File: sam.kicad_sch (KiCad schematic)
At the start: 59 parts, among them IC1 HYB4116, IC15 MC6883, IC16 74LS244N, IC2 HYB4116, IC3 HYB4116, IC31 74LS02N, IC33 74LS138N, IC4 HYB4116, IC5 HYB4116, IC6 HYB4116, IC7 HYB4116, IC8 HYB4116

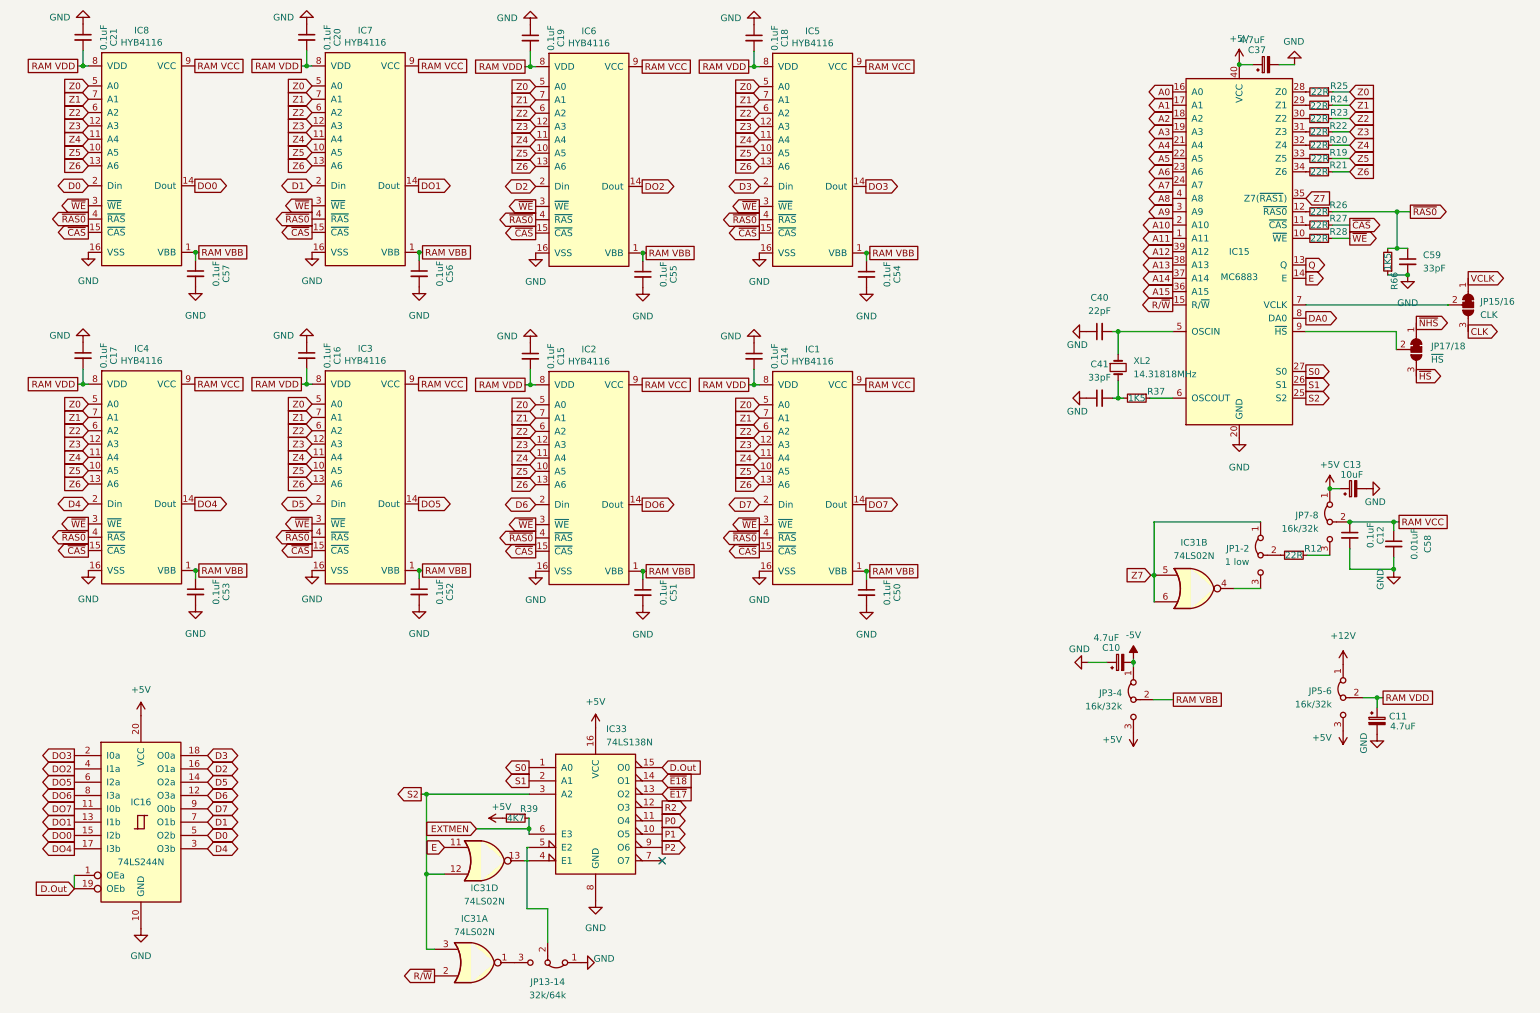
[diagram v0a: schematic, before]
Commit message: update board for revision 2.2
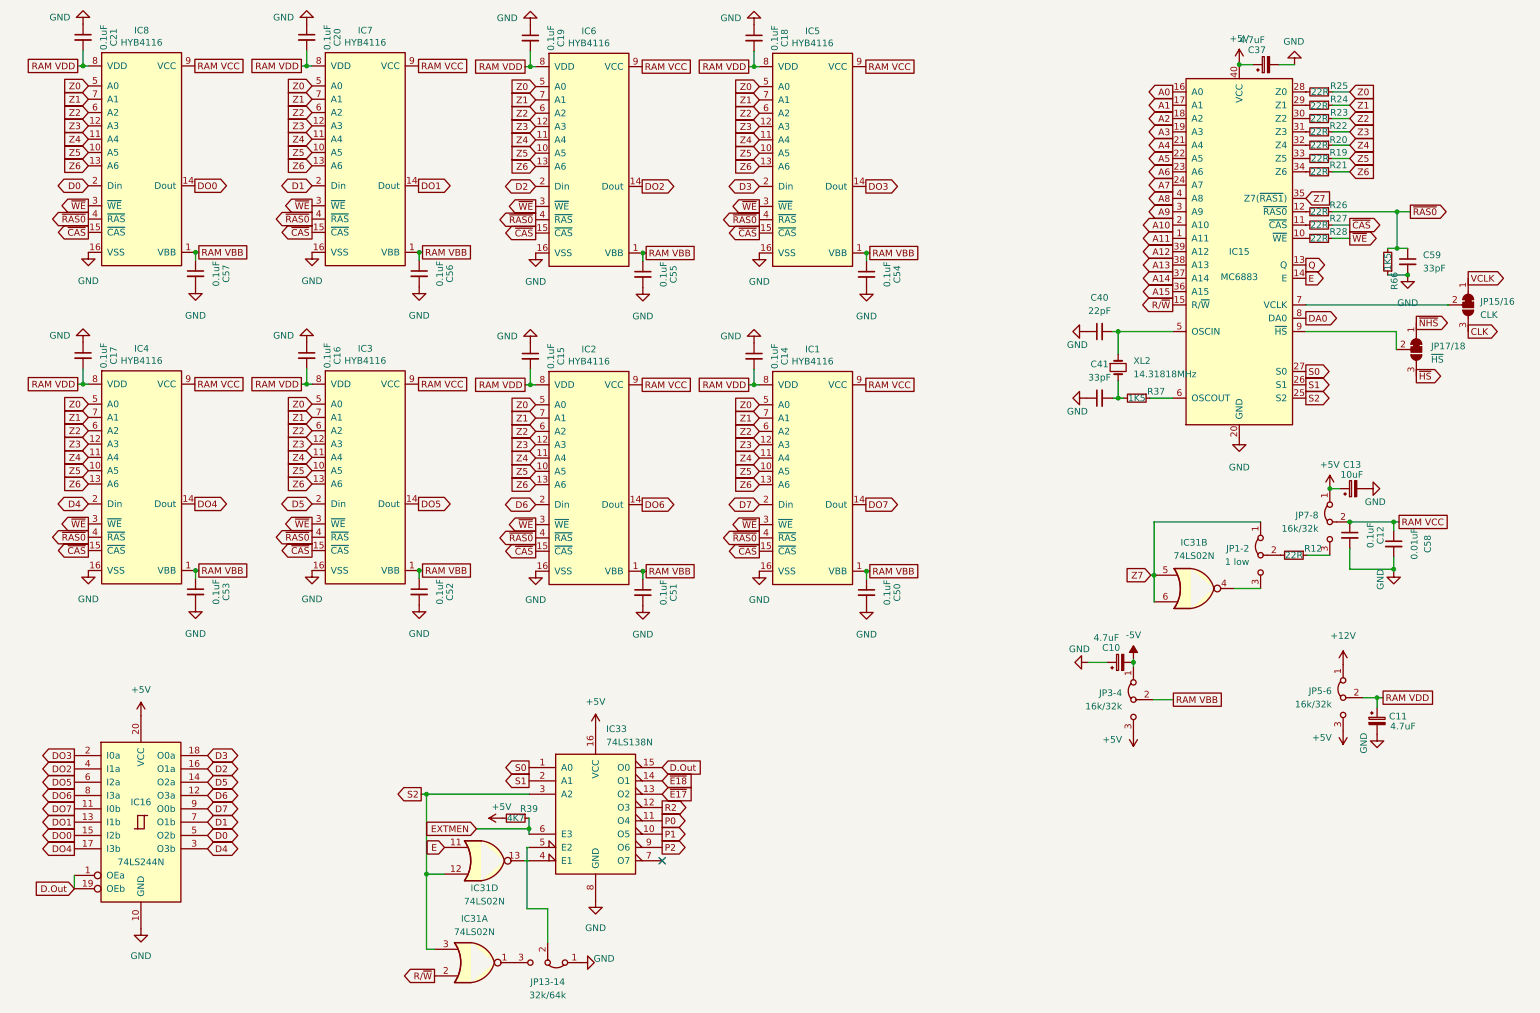
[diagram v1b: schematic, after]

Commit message: update bom references
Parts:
- IC1, IC2, IC3, IC4, IC5, IC6, IC7, IC8: Mouser (none) -> 517-4816-3000-CP
- IC15: Mouser (none) -> 517-4840-6000-CP
- JP1-2: DigiKey 952-2521-ND -> (none); Mouser (none) -> 538-22-28-5033
- JP13-14, JP3-4, JP5-6, JP7-8: Mouser (none) -> 538-22-28-5033
- JP15/16, JP17/18: now left out of the parts list
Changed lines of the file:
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@@
 			)
 		)
+		(property "Mouser" "517-4816-3000-CP"
+			(at 35.433 42.418 0)
+			(effects
+				(font
+					(size 1.27 1.27)
+				)
+				(hide yes)
+			)
+		)
 		(pin "1"
 		)
@@
 			)
 		)
+		(property "Mouser" "538-22-28-5033"
+			(at 112.903 195.707 0)
+			(effects
+				(font
+					(size 1.27 1.27)
+				)
+				(hide yes)
+			)
+		)
 		(pin "1"
 		)
@@
 			)
 		)
+		(property "Mouser" "517-4816-3000-CP"
+			(at 120.777 42.545 0)
+			(effects
+				(font
+					(size 1.27 1.27)
+				)
+				(hide yes)
+			)
+		)
 		(pin "1"
 		)
@@
 		(unit 1)
 		(exclude_from_sim no)
-		(in_bom yes)
+		(in_bom no)
 		(on_board yes)
 		(dnp no)
@@
 			)
 		)
+		(property "Mouser" "538-22-28-5033"
+			(at 264.668 145.161 90)
+			(effects
+				(font
+					(size 1.27 1.27)
+				)
+				(hide yes)
+			)
+		)
 		(pin "1"
 		)
@@
 			)
 		)
+		(property "Mouser" "517-4816-3000-CP"
+			(at 78.105 42.418 0)
+			(effects
+				(font
+					(size 1.27 1.27)
+				)
+				(hide yes)
+			)
+		)
 		(pin "1"
 		)
@@
 			)
 		)
+		(property "Mouser" "517-4816-3000-CP"
+			(at 120.777 103.251 0)
+			(effects
+				(font
+					(size 1.27 1.27)
+				)
+				(hide yes)
+			)
+		)
 		(pin "1"
 		)
@@
 			)
 		)
-		(property "DigiKey" "952-2521-ND"
+		(property "DigiKey" ""
 			(at 248.92 117.983 0)
 			(effects
@@
 			)
 		)
+		(property "Mouser" "538-22-28-5033"
+			(at 248.92 117.983 90)
+			(effects
+				(font
+					(size 1.27 1.27)
+				)
+				(hide yes)
+			)
+		)
 		(pin "1"
 		)
@@
 			)
 		)
+		(property "Mouser" "517-4816-3000-CP"
+			(at 35.433 103.124 0)
+			(effects
+				(font
+					(size 1.27 1.27)
+				)
+				(hide yes)
+			)
+		)
 		(pin "1"
 		)
@@
 			)
 		)
+		(property "Mouser" "517-4816-3000-CP"
+			(at 163.449 103.251 0)
+			(effects
+				(font
+					(size 1.27 1.27)
+				)
+				(hide yes)
+			)
+		)
 		(pin "1"
 		)
@@
 		(unit 1)
 		(exclude_from_sim no)
-		(in_bom yes)
+		(in_bom no)
 		(on_board yes)
 		(dnp no)
@@
 			)
 		)
+		(property "Mouser" "517-4816-3000-CP"
+			(at 163.449 42.545 0)
+			(effects
+				(font
+					(size 1.27 1.27)
+				)
+				(hide yes)
+			)
+		)
 		(pin "1"
 		)
@@
 			)
 		)
+		(property "Mouser" "517-4816-3000-CP"
+			(at 78.105 103.124 0)
+			(effects
+				(font
+					(size 1.27 1.27)
+				)
+				(hide yes)
+			)
+		)
 		(pin "1"
 		)
@@
 			)
 		)
+		(property "Mouser" "538-22-28-5033"
+			(at 262.128 111.633 90)
+			(effects
+				(font
+					(size 1.27 1.27)
+				)
+				(hide yes)
+			)
+		)
 		(pin "1"
 		)
@@
 			)
 		)
+		(property "Mouser" "517-4840-6000-CP"
+			(at 244.856 60.071 0)
+			(effects
+				(font
+					(size 1.27 1.27)
+				)
+				(hide yes)
+			)
+		)
 		(pin "1"
 		)
@@
 			(effects
 				(font
+					(size 1.27 1.27)
+				)
+				(hide yes)
+			)
+		)
+		(property "Mouser" "538-22-28-5033"
+			(at 224.663 145.542 90)
+			(effects
+				(font
